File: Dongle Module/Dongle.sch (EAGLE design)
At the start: 29 parts, among them Q2 2.5A/30V, U1 RFM69HCW, U10 74AHC1G125, U8 ATSAMD21G-A, U9 3.3V, Y1 32.768kHz

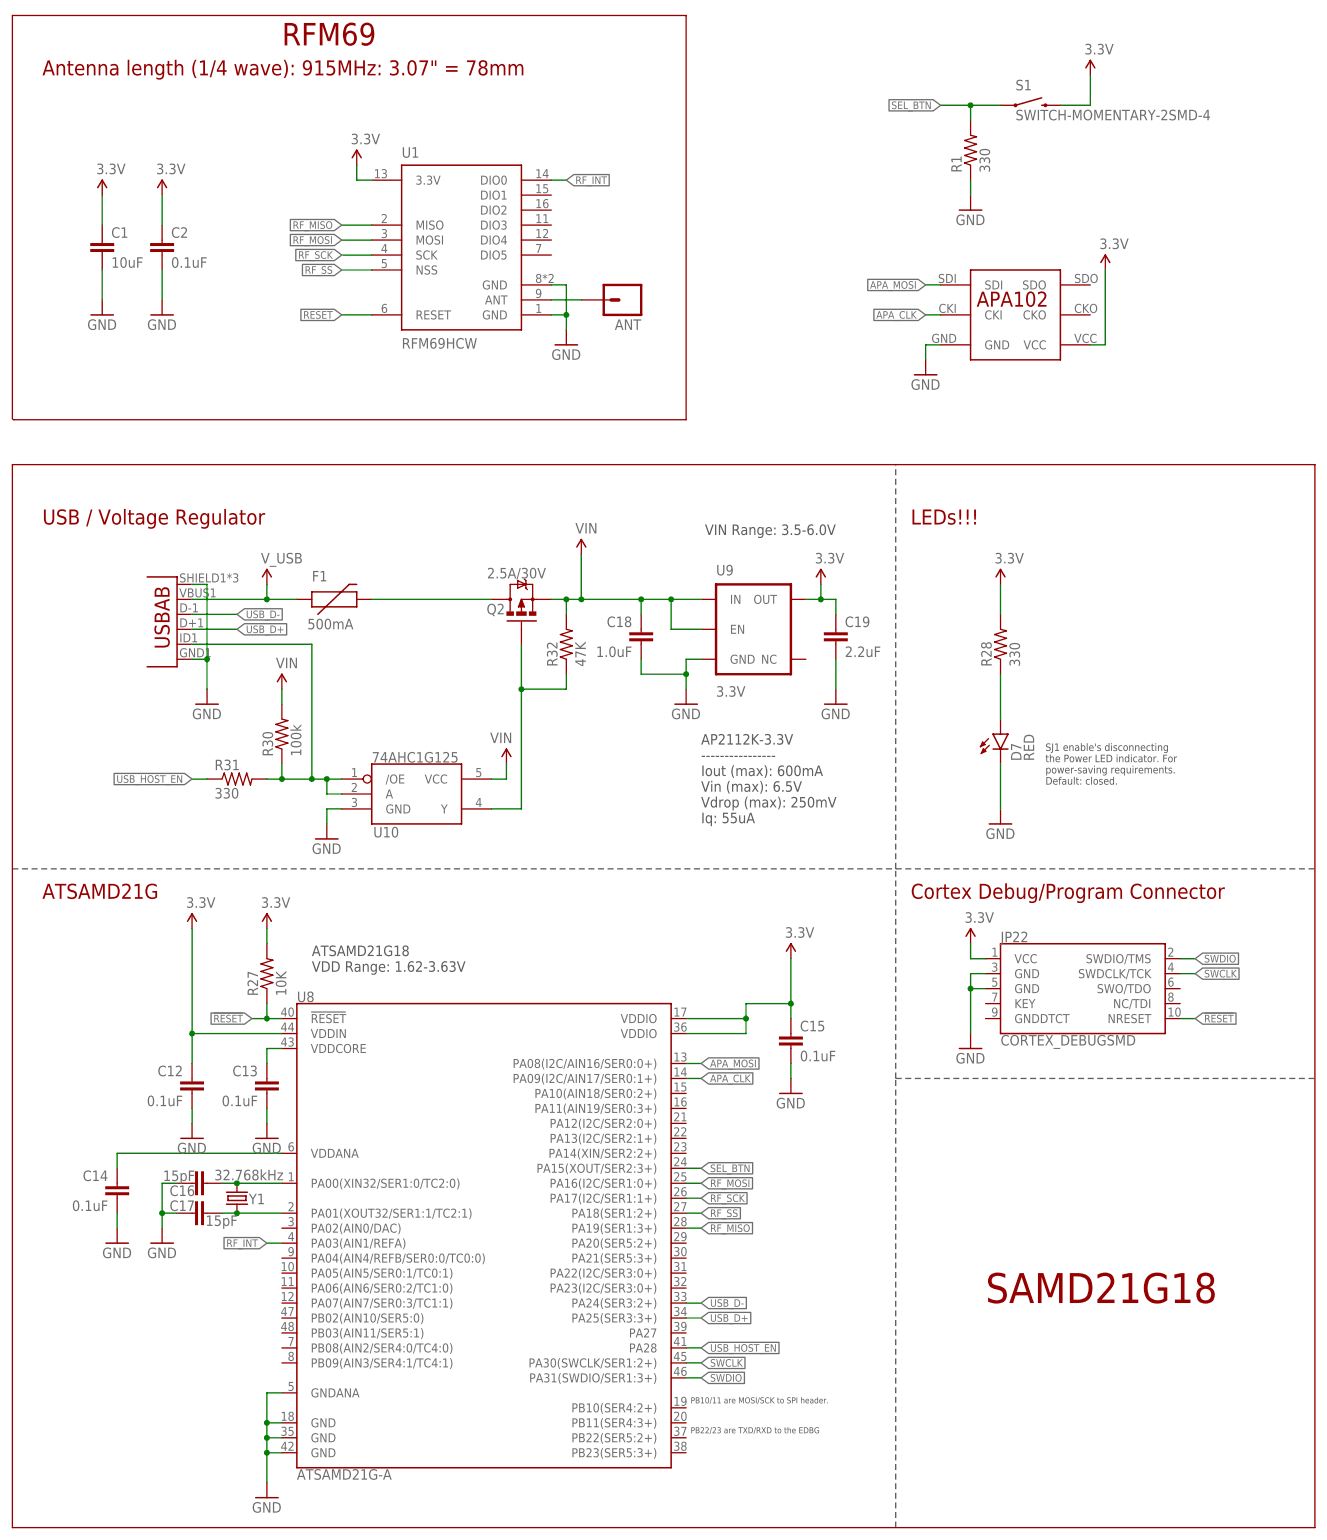
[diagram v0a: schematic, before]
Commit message: Finalized all PCBs
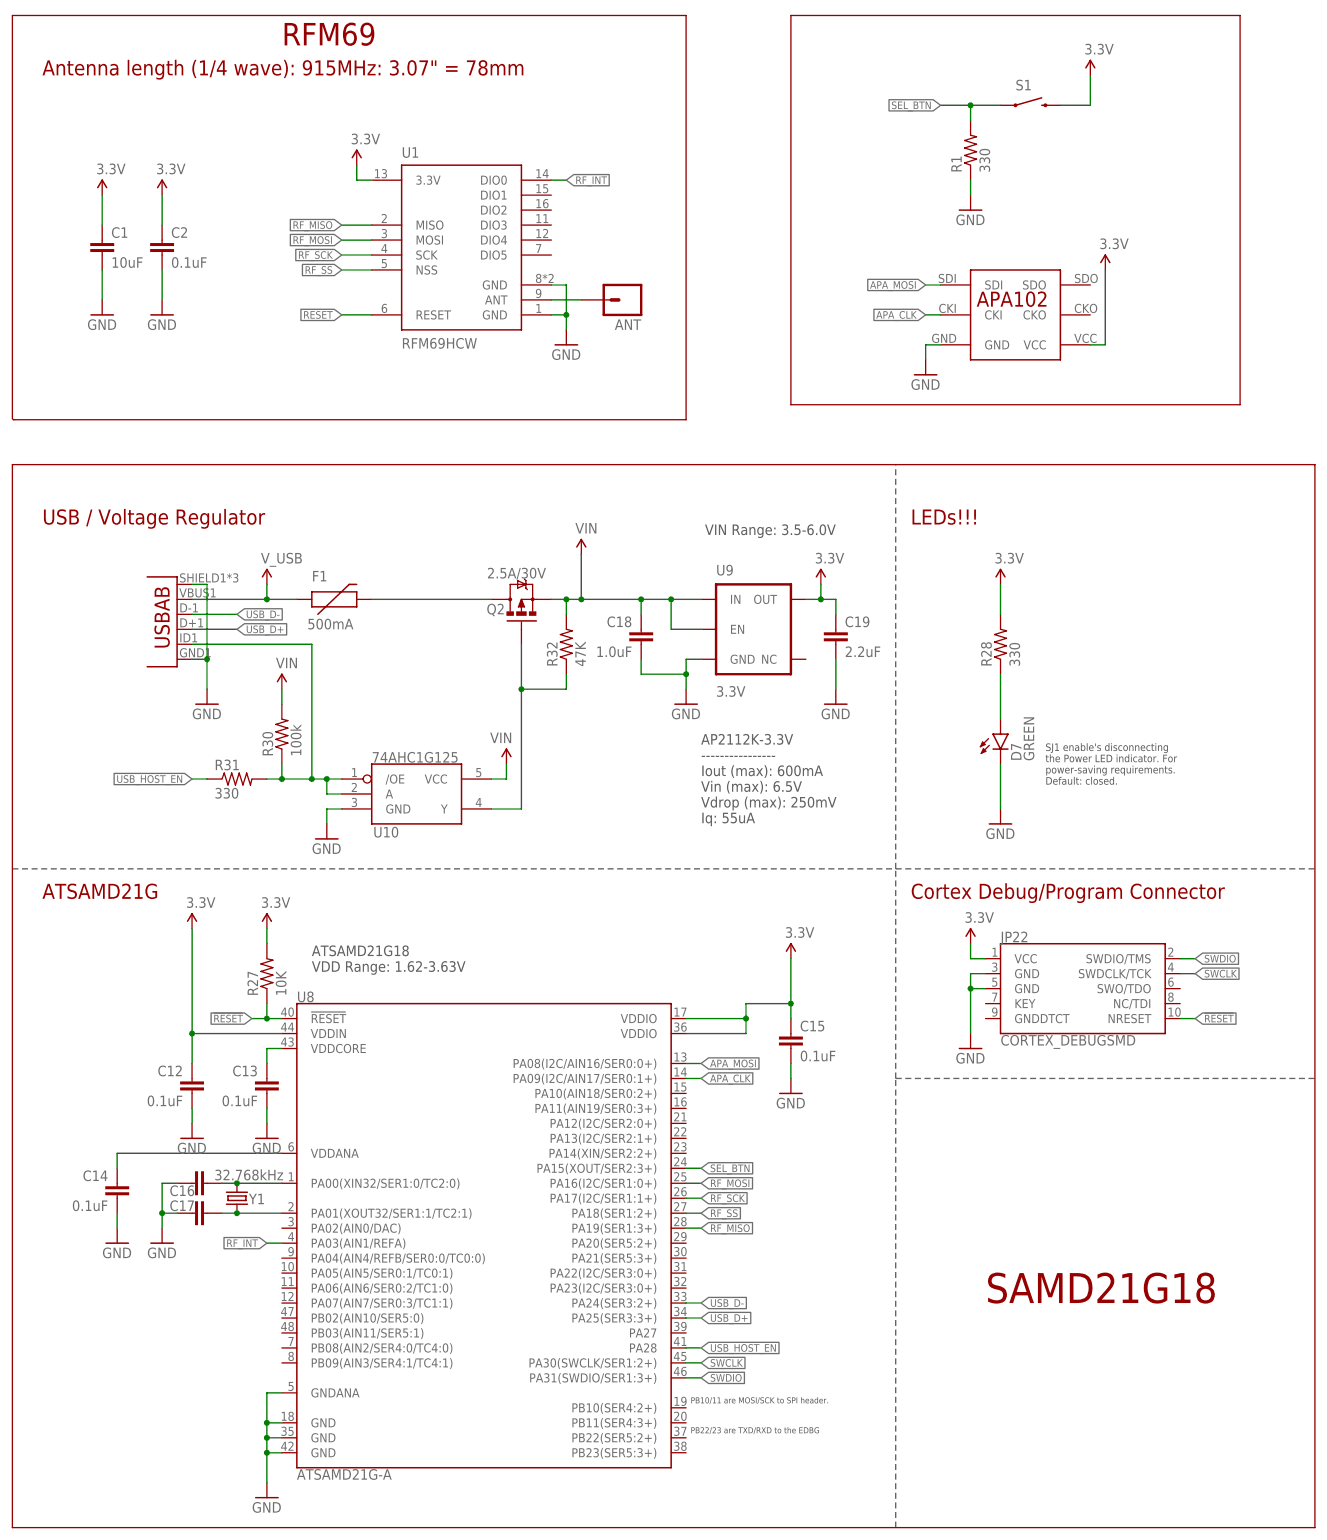
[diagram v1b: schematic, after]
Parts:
- C12, C13, C14, C15: device SparkFun-Capacitors:0.1UF-16V(+-10%)(0402) -> SparkFun-Capacitors:CAP0603-CAP
- C16, C17: device samd21-temp:15PF-50V(+-5%)(0402) -> SparkFun-Capacitors:CAP0603-CAP
- D7: value RED -> GREEN
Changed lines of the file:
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@@
 <part name="U8" library="samd21-temp" deviceset="ATSAMD21G" device="-A"/>
 <part name="GND40" library="SparkFun-Aesthetics" deviceset="GND" device=""/>
-<part name="C12" library="SparkFun-Capacitors" deviceset="0.1UF-16V(+-10%)(0402)" device="" value="0.1uF"/>
-<part name="C13" library="SparkFun-Capacitors" deviceset="0.1UF-16V(+-10%)(0402)" device="" value="0.1uF"/>
-<part name="C14" library="SparkFun-Capacitors" deviceset="0.1UF-16V(+-10%)(0402)" device="" value="0.1uF"/>
-<part name="C15" library="SparkFun-Capacitors" deviceset="0.1UF-16V(+-10%)(0402)" device="" value="0.1uF"/>
+<part name="C12" library="SparkFun-Capacitors" deviceset="CAP" device="0603-CAP" value="0.1uF"/>
+<part name="C13" library="SparkFun-Capacitors" deviceset="CAP" device="0603-CAP" value="0.1uF"/>
+<part name="C14" library="SparkFun-Capacitors" deviceset="CAP" device="0603-CAP" value="0.1uF"/>
+<part name="C15" library="SparkFun-Capacitors" deviceset="CAP" device="0603-CAP" value="0.1uF"/>
 <part name="R27" library="SparkFun-Resistors" deviceset="10KOHM-1/10W-1%(0603)" device="0603" value="10K"/>
 <part name="SUPPLY12" library="SparkFun-Aesthetics" deviceset="3.3V" device=""/>
@@
 <part name="GND42" library="SparkFun-Aesthetics" deviceset="GND" device=""/>
 <part name="GND43" library="SparkFun-Aesthetics" deviceset="GND" device=""/>
-<part name="C16" library="samd21-temp" deviceset="15PF-50V(+-5%)(0402)" device="" value="15pF"/>
-<part name="C17" library="samd21-temp" deviceset="15PF-50V(+-5%)(0402)" device="" value="15pF"/>
+<part name="C16" library="SparkFun-Capacitors" deviceset="CAP" device="0603-CAP" value="15pF"/>
+<part name="C17" library="SparkFun-Capacitors" deviceset="CAP" device="0603-CAP" value="15pF"/>
 <part name="GND44" library="SparkFun-Aesthetics" deviceset="GND" device=""/>
 <part name="SUPPLY15" library="SparkFun-Aesthetics" deviceset="3.3V" device=""/>
@@
 <part name="GND49" library="SparkFun-Aesthetics" deviceset="GND" device=""/>
 <part name="SUPPLY16" library="SparkFun-Aesthetics" deviceset="3.3V" device=""/>
-<part name="D7" library="SparkFun-LED" deviceset="LED-RED" device="0603" value="RED"/>
+<part name="D7" library="SparkFun-LED" deviceset="LED-RED" device="0603" value="GREEN"/>
 <part name="R28" library="SparkFun-Resistors" deviceset="330OHM1/10W1%(0603)" device="" value="330"/>
 <part name="SUPPLY17" library="SparkFun-Aesthetics" deviceset="3.3V" device=""/>
@@
 <wire x1="0" y1="0" x2="0" y2="180.34" width="0.1524" layer="94"/>
 <text x="165.1" y="38.1" size="5.08" layer="94" ratio="15">SAMD21G18</text>
+<wire x1="132.08" y1="256.54" x2="208.28" y2="256.54" width="0.1524" layer="94"/>
+<wire x1="208.28" y1="256.54" x2="208.28" y2="190.5" width="0.1524" layer="94"/>
+<wire x1="208.28" y1="190.5" x2="132.08" y2="190.5" width="0.1524" layer="94"/>
+<wire x1="132.08" y1="190.5" x2="132.08" y2="256.54" width="0.1524" layer="94"/>
 </plain>
 <instances>
@@
 <instance part="C16" gate="G$1" x="33.02" y="58.42" smashed="yes" rot="R90">
 <attribute name="NAME" x="30.988" y="58.039" size="1.778" layer="95" rot="R180"/>
-<attribute name="VALUE" x="30.988" y="58.801" size="1.778" layer="96" rot="MR0"/>
 </instance>
 <instance part="C17" gate="G$1" x="30.48" y="53.34" smashed="yes" rot="R270">
 <attribute name="NAME" x="30.988" y="53.721" size="1.778" layer="95" rot="MR0"/>
-<attribute name="VALUE" x="32.766" y="52.959" size="1.778" layer="96" rot="MR180"/>
 </instance>
 <instance part="GND44" gate="1" x="25.4" y="48.26"/>
@@
 <instance part="SUPPLY24" gate="G$1" x="96.52" y="165.1"/>
 <instance part="SUPPLY18" gate="G$1" x="43.18" y="160.02"/>
-<instance part="S1" gate="G$1" x="172.72" y="241.3"/>
+<instance part="S1" gate="G$1" x="172.72" y="241.3" smashed="yes">
+<attribute name="NAME" x="170.18" y="243.84" size="1.778" layer="95"/>
+</instance>
 <instance part="SUPPLY3" gate="G$1" x="182.88" y="246.38"/>
 <instance part="GND4" gate="1" x="162.56" y="223.52"/>

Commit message: push ui.c again
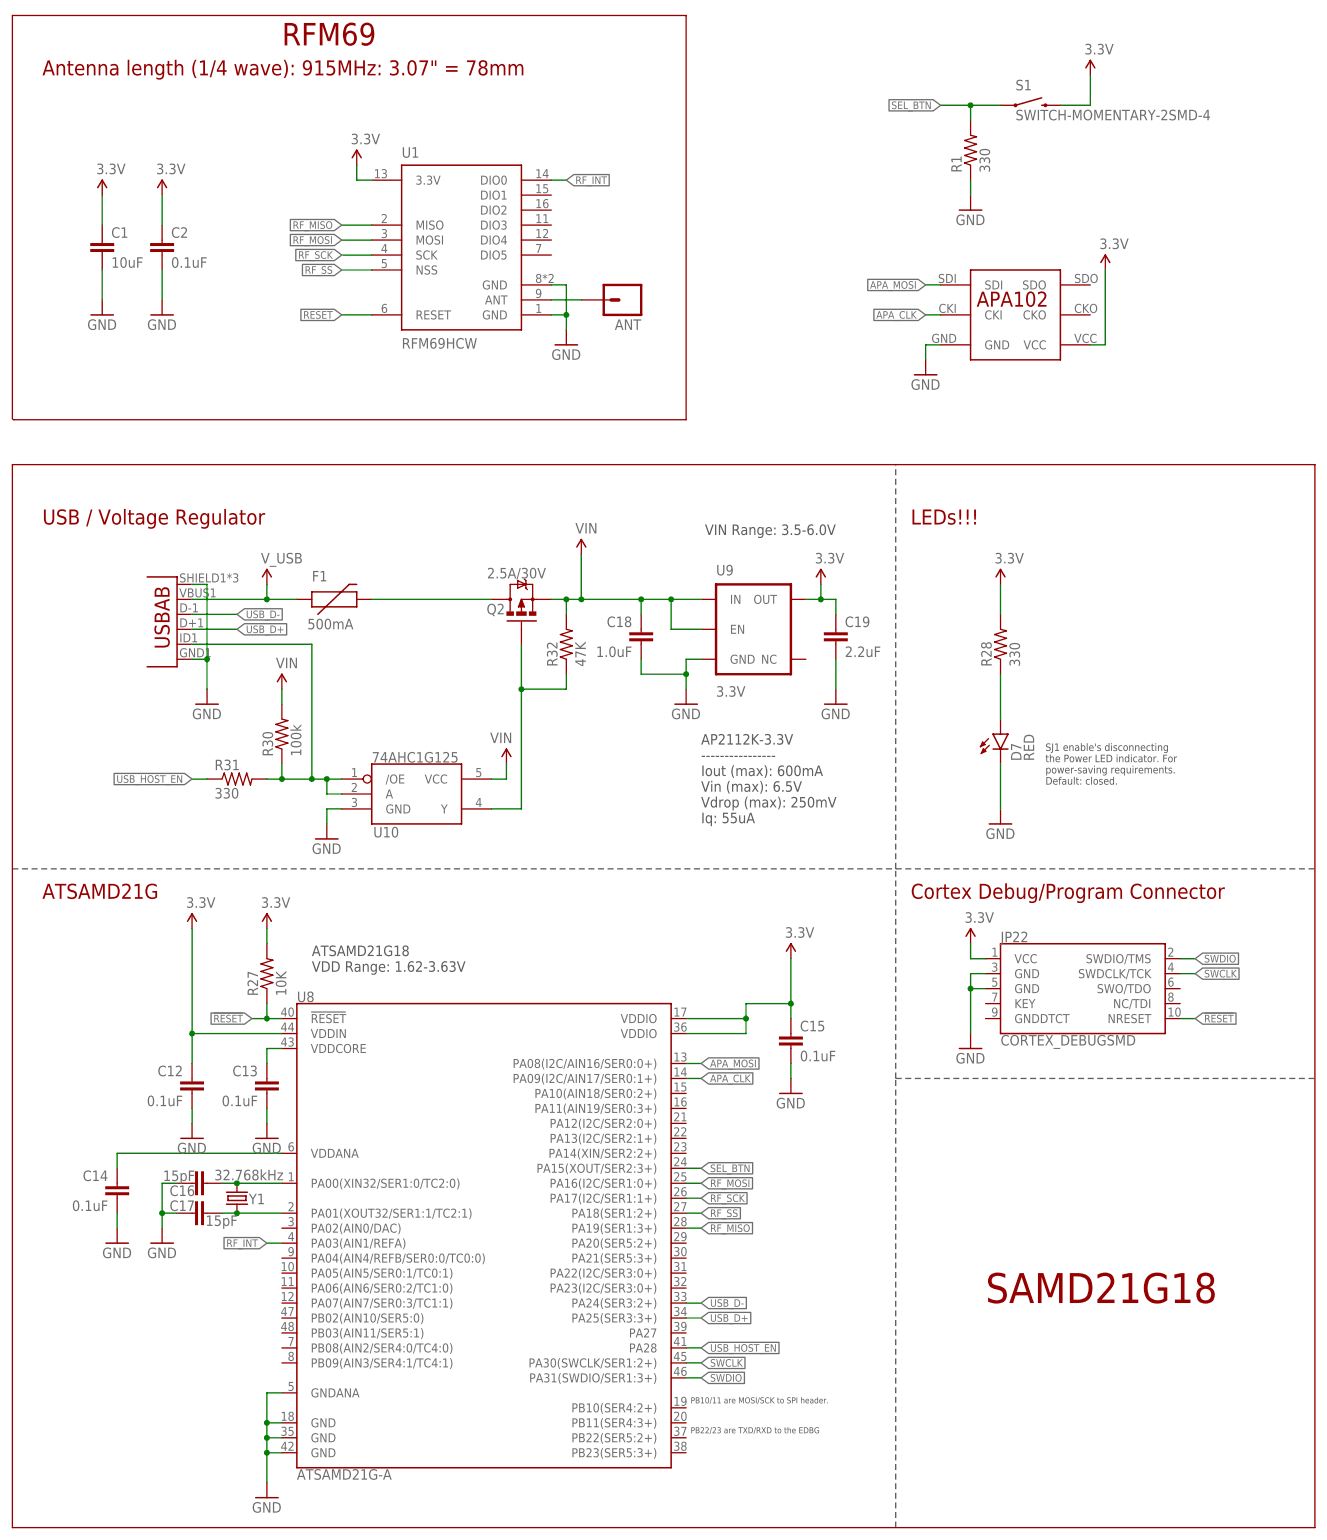
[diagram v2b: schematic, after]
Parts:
- C12, C13, C14, C15: device SparkFun-Capacitors:CAP0603-CAP -> SparkFun-Capacitors:0.1UF-16V(+-10%)(0402)
- C16, C17: device SparkFun-Capacitors:CAP0603-CAP -> samd21-temp:15PF-50V(+-5%)(0402)
- D7: value GREEN -> RED
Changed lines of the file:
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@@
 <part name="U8" library="samd21-temp" deviceset="ATSAMD21G" device="-A"/>
 <part name="GND40" library="SparkFun-Aesthetics" deviceset="GND" device=""/>
-<part name="C12" library="SparkFun-Capacitors" deviceset="CAP" device="0603-CAP" value="0.1uF"/>
-<part name="C13" library="SparkFun-Capacitors" deviceset="CAP" device="0603-CAP" value="0.1uF"/>
-<part name="C14" library="SparkFun-Capacitors" deviceset="CAP" device="0603-CAP" value="0.1uF"/>
-<part name="C15" library="SparkFun-Capacitors" deviceset="CAP" device="0603-CAP" value="0.1uF"/>
+<part name="C12" library="SparkFun-Capacitors" deviceset="0.1UF-16V(+-10%)(0402)" device="" value="0.1uF"/>
+<part name="C13" library="SparkFun-Capacitors" deviceset="0.1UF-16V(+-10%)(0402)" device="" value="0.1uF"/>
+<part name="C14" library="SparkFun-Capacitors" deviceset="0.1UF-16V(+-10%)(0402)" device="" value="0.1uF"/>
+<part name="C15" library="SparkFun-Capacitors" deviceset="0.1UF-16V(+-10%)(0402)" device="" value="0.1uF"/>
 <part name="R27" library="SparkFun-Resistors" deviceset="10KOHM-1/10W-1%(0603)" device="0603" value="10K"/>
 <part name="SUPPLY12" library="SparkFun-Aesthetics" deviceset="3.3V" device=""/>
@@
 <part name="GND42" library="SparkFun-Aesthetics" deviceset="GND" device=""/>
 <part name="GND43" library="SparkFun-Aesthetics" deviceset="GND" device=""/>
-<part name="C16" library="SparkFun-Capacitors" deviceset="CAP" device="0603-CAP" value="15pF"/>
-<part name="C17" library="SparkFun-Capacitors" deviceset="CAP" device="0603-CAP" value="15pF"/>
+<part name="C16" library="samd21-temp" deviceset="15PF-50V(+-5%)(0402)" device="" value="15pF"/>
+<part name="C17" library="samd21-temp" deviceset="15PF-50V(+-5%)(0402)" device="" value="15pF"/>
 <part name="GND44" library="SparkFun-Aesthetics" deviceset="GND" device=""/>
 <part name="SUPPLY15" library="SparkFun-Aesthetics" deviceset="3.3V" device=""/>
@@
 <part name="GND49" library="SparkFun-Aesthetics" deviceset="GND" device=""/>
 <part name="SUPPLY16" library="SparkFun-Aesthetics" deviceset="3.3V" device=""/>
-<part name="D7" library="SparkFun-LED" deviceset="LED-RED" device="0603" value="GREEN"/>
+<part name="D7" library="SparkFun-LED" deviceset="LED-RED" device="0603" value="RED"/>
 <part name="R28" library="SparkFun-Resistors" deviceset="330OHM1/10W1%(0603)" device="" value="330"/>
 <part name="SUPPLY17" library="SparkFun-Aesthetics" deviceset="3.3V" device=""/>
@@
 <wire x1="0" y1="0" x2="0" y2="180.34" width="0.1524" layer="94"/>
 <text x="165.1" y="38.1" size="5.08" layer="94" ratio="15">SAMD21G18</text>
-<wire x1="132.08" y1="256.54" x2="208.28" y2="256.54" width="0.1524" layer="94"/>
-<wire x1="208.28" y1="256.54" x2="208.28" y2="190.5" width="0.1524" layer="94"/>
-<wire x1="208.28" y1="190.5" x2="132.08" y2="190.5" width="0.1524" layer="94"/>
-<wire x1="132.08" y1="190.5" x2="132.08" y2="256.54" width="0.1524" layer="94"/>
 </plain>
 <instances>
@@
 <instance part="C16" gate="G$1" x="33.02" y="58.42" smashed="yes" rot="R90">
 <attribute name="NAME" x="30.988" y="58.039" size="1.778" layer="95" rot="R180"/>
+<attribute name="VALUE" x="30.988" y="58.801" size="1.778" layer="96" rot="MR0"/>
 </instance>
 <instance part="C17" gate="G$1" x="30.48" y="53.34" smashed="yes" rot="R270">
 <attribute name="NAME" x="30.988" y="53.721" size="1.778" layer="95" rot="MR0"/>
+<attribute name="VALUE" x="32.766" y="52.959" size="1.778" layer="96" rot="MR180"/>
 </instance>
 <instance part="GND44" gate="1" x="25.4" y="48.26"/>
@@
 <instance part="SUPPLY24" gate="G$1" x="96.52" y="165.1"/>
 <instance part="SUPPLY18" gate="G$1" x="43.18" y="160.02"/>
-<instance part="S1" gate="G$1" x="172.72" y="241.3" smashed="yes">
-<attribute name="NAME" x="170.18" y="243.84" size="1.778" layer="95"/>
-</instance>
+<instance part="S1" gate="G$1" x="172.72" y="241.3"/>
 <instance part="SUPPLY3" gate="G$1" x="182.88" y="246.38"/>
 <instance part="GND4" gate="1" x="162.56" y="223.52"/>
